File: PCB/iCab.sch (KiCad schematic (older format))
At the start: 56 parts, among them J1 Jack-DC, J10 PORT5, J11 V12, J2 Jack-DC, J3 PGM, J4 SERIAL, J5 PORT1, J6 PORT2, J7 OUT, J8 PORT3, J9 PORT4, Q1 IRFZ44, Q2 IRFZ44, Q3 IRFZ44, Q4 IRFZ44, Q5 IRFZ44, SW1 SW_Push, U1 Output, U2 PIC18F2550, U3 Output, Y1 Crystal

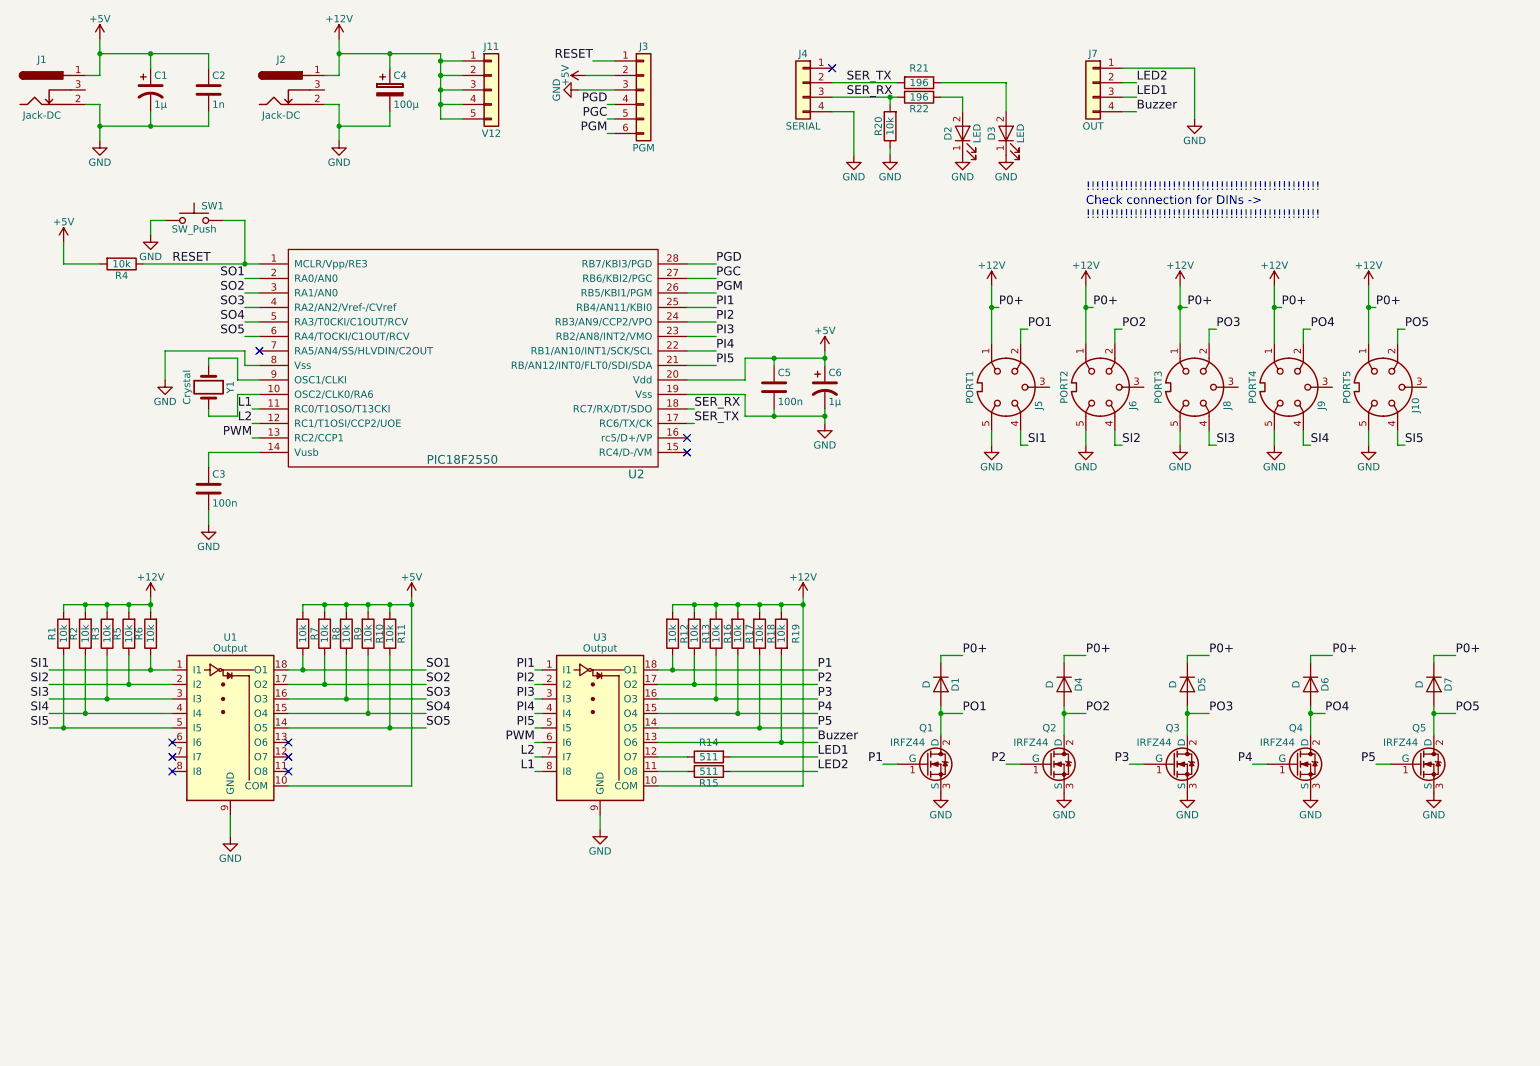
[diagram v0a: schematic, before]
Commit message: new pcb
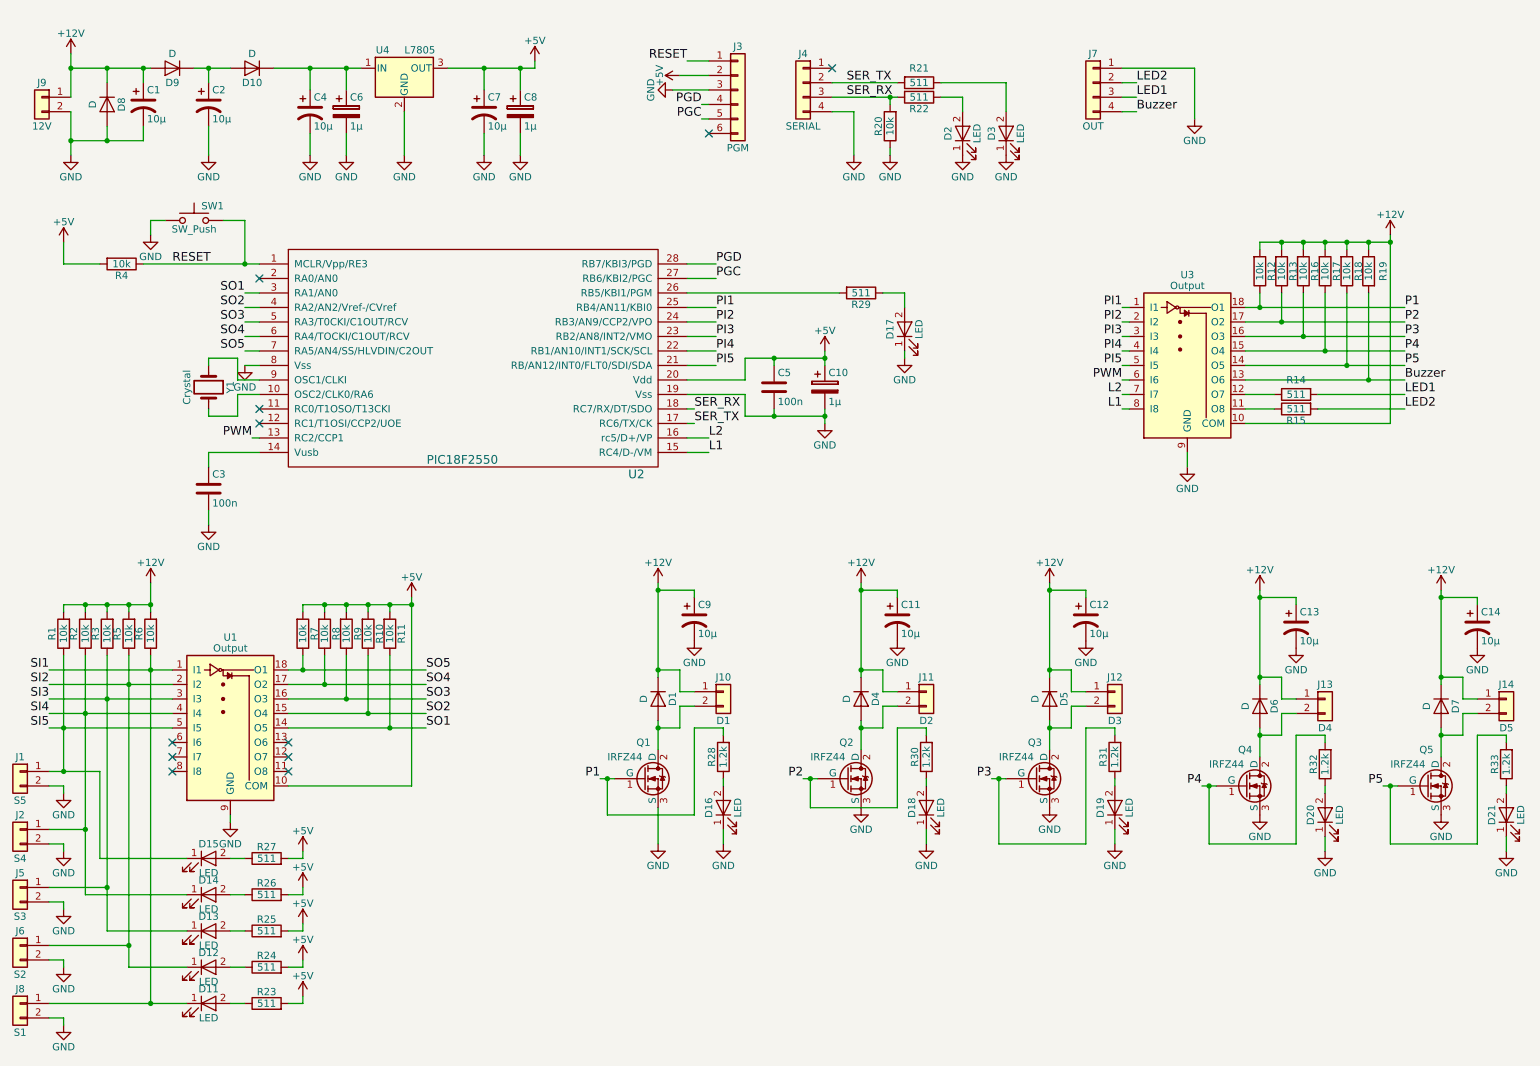
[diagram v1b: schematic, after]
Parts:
- removed C2: 1n, Capacitors_SMD:C_0603_HandSoldering, symbol C
- removed C4: 100µ, Capacitors_THT:CP_Radial_D10.0mm_P5.00mm, symbol CP
- removed C6: 1µ, Capacitors_Tantalum_SMD:CP_Tantalum_Case-A_EIA-3216-18_Reflow, symbol CP1
- removed J1, J2: Jack-DC, Connectors:BARREL_JACK, symbol Jack-DC
- removed J10: PORT5, Pin_Headers:Pin_Header_Straight_1x05_Pitch2.54mm, symbol DIN-5
- removed J11: V12, Pin_Headers:Pin_Header_Straight_1x05_Pitch2.54mm, symbol Conn_01x05
- removed J5: PORT1, Pin_Headers:Pin_Header_Straight_1x05_Pitch2.54mm, symbol DIN-5
- removed J6: PORT2, Pin_Headers:Pin_Header_Straight_1x05_Pitch2.54mm, symbol DIN-5
- removed J8: PORT3, Pin_Headers:Pin_Header_Straight_1x05_Pitch2.54mm, symbol DIN-5
- removed J9: PORT4, Pin_Headers:Pin_Header_Straight_1x05_Pitch2.54mm, symbol DIN-5
- added C10, C6, C8: 1µ, Capacitors_Tantalum_SMD:CP_Tantalum_Case-A_EIA-3216-18_Reflow, symbol CP
- added C11, C12, C13, C14, C2, C4, C7, C9: 10µ, Capacitors_THT:CP_Radial_D5.0mm_P2.00mm, symbol CP1
- added D10, D8, D9: D, Diodes_THT:D_T-1_P10.16mm_Horizontal, symbol D
- added D11, D12, D13, D14, D15, D16, D17, D18, D19, D20, D21: LED, LEDs:LED_0603_HandSoldering, symbol LED
- added J1: S5, TerminalBlock_Phoenix:TerminalBlock_Phoenix_MKDS-1,5-2_1x02_P5.00mm_Horizontal, symbol Conn_01x02
- added J10: D1, TerminalBlock_Phoenix:TerminalBlock_Phoenix_MKDS-1,5-2_1x02_P5.00mm_Horizontal, symbol Conn_01x02
- added J11: D2, TerminalBlock_Phoenix:TerminalBlock_Phoenix_MKDS-1,5-2_1x02_P5.00mm_Horizontal, symbol Conn_01x02
- added J12: D3, TerminalBlock_Phoenix:TerminalBlock_Phoenix_MKDS-1,5-2_1x02_P5.00mm_Horizontal, symbol Conn_01x02
- added J13: D4, TerminalBlock_Phoenix:TerminalBlock_Phoenix_MKDS-1,5-2_1x02_P5.00mm_Horizontal, symbol Conn_01x02
- added J14: D5, TerminalBlock_Phoenix:TerminalBlock_Phoenix_MKDS-1,5-2_1x02_P5.00mm_Horizontal, symbol Conn_01x02
- added J2: S4, TerminalBlock_Phoenix:TerminalBlock_Phoenix_MKDS-1,5-2_1x02_P5.00mm_Horizontal, symbol Conn_01x02
- added J5: S3, TerminalBlock_Phoenix:TerminalBlock_Phoenix_MKDS-1,5-2_1x02_P5.00mm_Horizontal, symbol Conn_01x02
- added J6: S2, TerminalBlock_Phoenix:TerminalBlock_Phoenix_MKDS-1,5-2_1x02_P5.00mm_Horizontal, symbol Conn_01x02
- added J8: S1, TerminalBlock_Phoenix:TerminalBlock_Phoenix_MKDS-1,5-2_1x02_P5.00mm_Horizontal, symbol Conn_01x02
- added J9: 12V, TerminalBlock_Phoenix:TerminalBlock_Phoenix_MKDS-1,5-2_1x02_P5.00mm_Horizontal, symbol Conn_01x02
- added R23, R24, R25, R26, R27, R29: 511, Resistors_SMD:R_0603_HandSoldering, symbol R
- added R28, R30, R31, R32, R33: 1.2k, Resistors_SMD:R_0603_HandSoldering, symbol R
- added U4: L7805, TO_SOT_Packages_THT:TO-220_Vertical, symbol L7805
- C1: value 1µ -> 10µ; footprint Capacitors_Tantalum_SMD:CP_Tantalum_Case-A_EIA-3216-18_Reflow -> Capacitors_THT:CP_Radial_D5.0mm_P2.00mm
- D1, D4, D5, D6, D7: footprint Diodes_SMD:D_MELF_Handsoldering -> Diodes_THT:D_T-1_P5.08mm_Horizontal
- J3: footprint Pin_Headers:Pin_Header_Angled_1x06_Pitch2.54mm -> Pin_Headers:Pin_Header_Straight_1x06_Pitch2.54mm
- R21, R22: value 196 -> 511
- SW1: footprint Buttons_Switches_SMD:SW_SPST_KMR2 -> Buttons_Switches_THT:SW_PUSH_6mm
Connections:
- net +12V: now also C1.1, C11.1, C12.1, C13.1, C14.1, C9.1, D8.1 (K), D9.2 (A), J10.1 (Pin_1), J11.1 (Pin_1), J12.1 (Pin_1), J13.1 (Pin_1), J14.1 (Pin_1), J9.1 (Pin_1)
- net +5V: now also C10.1, C7.1, C8.1, R23.2, R24.2, R25.2, R26.2, R27.2, U4.3 (OUT); no longer C1.1
- net GND: now also C10.2, C11.2, C12.2, C13.2, C14.2, C2.2, C4.2, C6.2, C7.2, C8.2, C9.2, D16.1 (K), D17.1 (K), D18.1 (K), D19.1 (K), D20.1 (K), D21.1 (K), D8.2 (A), J1.2 (Pin_2), J2.2 (Pin_2), J5.2 (Pin_2), J6.2 (Pin_2), J8.2 (Pin_2), J9.2 (Pin_2), U4.2 (GND)
- net L1: now also U2.15 (RC4/D-/VM); no longer U2.11 (RC0/T1OSO/T13CKI)
- net L2: now also U2.16 (rc5/D+/VP); no longer U2.12 (RC1/T1OSI/CCP2/UOE)
- net P1: now also R28.2
- net P2: now also R30.2
- net P3: now also R31.2
- net P4: now also R32.2
- net P5: now also R33.2
- net SI1: now also D11.1 (K), J8.1 (Pin_1)
- net SI2: now also D12.1 (K), J6.1 (Pin_1)
- net SI3: now also D13.1 (K), J5.1 (Pin_1)
- net SI4: now also D14.1 (K), J2.1 (Pin_1)
- net SI5: now also D15.1 (K), J1.1 (Pin_1)
- net SO1: now also R11.1, U1.14 (O5), U2.3 (RA1/AN0); no longer R7.1, U1.18 (O1), U2.2 (RA0/AN0)
- net SO2: now also R10.1, U1.15 (O4), U2.4 (RA2/AN2/Vref-/CVref); no longer R8.1, U1.17 (O2), U2.3 (RA1/AN0)
- net SO3: now also U2.5 (RA3/T0CKI/C1OUT/RCV); no longer U2.4 (RA2/AN2/Vref-/CVref)
- net SO4: now also R8.1, U1.17 (O2), U2.6 (RA4/TOCKI/C1OUT/RCV); no longer R10.1, U1.15 (O4), U2.5 (RA3/T0CKI/C1OUT/RCV)
- net SO5: now also R7.1, U1.18 (O1), U2.7 (RA5/AN4/SS/HLVDIN/C2OUT); no longer R11.1, U1.14 (O5), U2.6 (RA4/TOCKI/C1OUT/RCV)
- net PGM: no longer names the net of U2.26 (RB5/KBI1/PGM)
- net PGM: now also R29.2; no longer J3.6 (Pin_6)
- net PO1: no longer names the net of D1.2 (A), Q1.2 (D)
- net PO1: now also J10.2 (Pin_2)
- net PO2: no longer names the net of D4.2 (A), Q2.2 (D)
- net PO2: now also J11.2 (Pin_2)
- net PO3: no longer names the net of D5.2 (A), Q3.2 (D)
- net PO3: now also J12.2 (Pin_2)
- net PO4: no longer names the net of D6.2 (A), Q4.2 (D)
- net PO4: now also J13.2 (Pin_2)
- net PO5: no longer names the net of D7.2 (A), Q5.2 (D)
- net PO5: now also J14.2 (Pin_2)
- new net: D17.2 (A), R29.1
- new net: D16.2 (A), R28.1
- new net: D18.2 (A), R30.1
- new net: D19.2 (A), R31.1
- new net: D20.2 (A), R32.1
- new net: D21.2 (A), R33.1
- new net: D11.2 (A), R23.1
- new net: D12.2 (A), R24.1
- new net: D13.2 (A), R25.1
- new net: D14.2 (A), R26.1
- new net: D15.2 (A), R27.1
- new net: C2.1, D10.2 (A), D9.1 (K)
- new net: C4.1, C6.1, D10.1 (K), U4.1 (IN)
- no-connect marks 10 -> 11
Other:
- note removed: "!!!!!!!!!!!!!!!!!!!!!!!!!!!!!!!!!!!!!!!!!!!!!!!!!\nCheck connection for DINs ->\n!!!!!!!!!!!!!!!!!!!!!!!!!!!!!!!!!!!!!!!!!!!!!!!!!"
- moved on the sheet: D1, D4, D5, D6, D7, J3, Q1, Q2, Q3, Q4, Q5, R12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
